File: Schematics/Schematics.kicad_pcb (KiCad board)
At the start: 2 copper layers, 104.1 x 68.6 mm, 15 parts, among them SW1 SW_MEC_5E, U1 74HC595, U2 CC56-12YWA

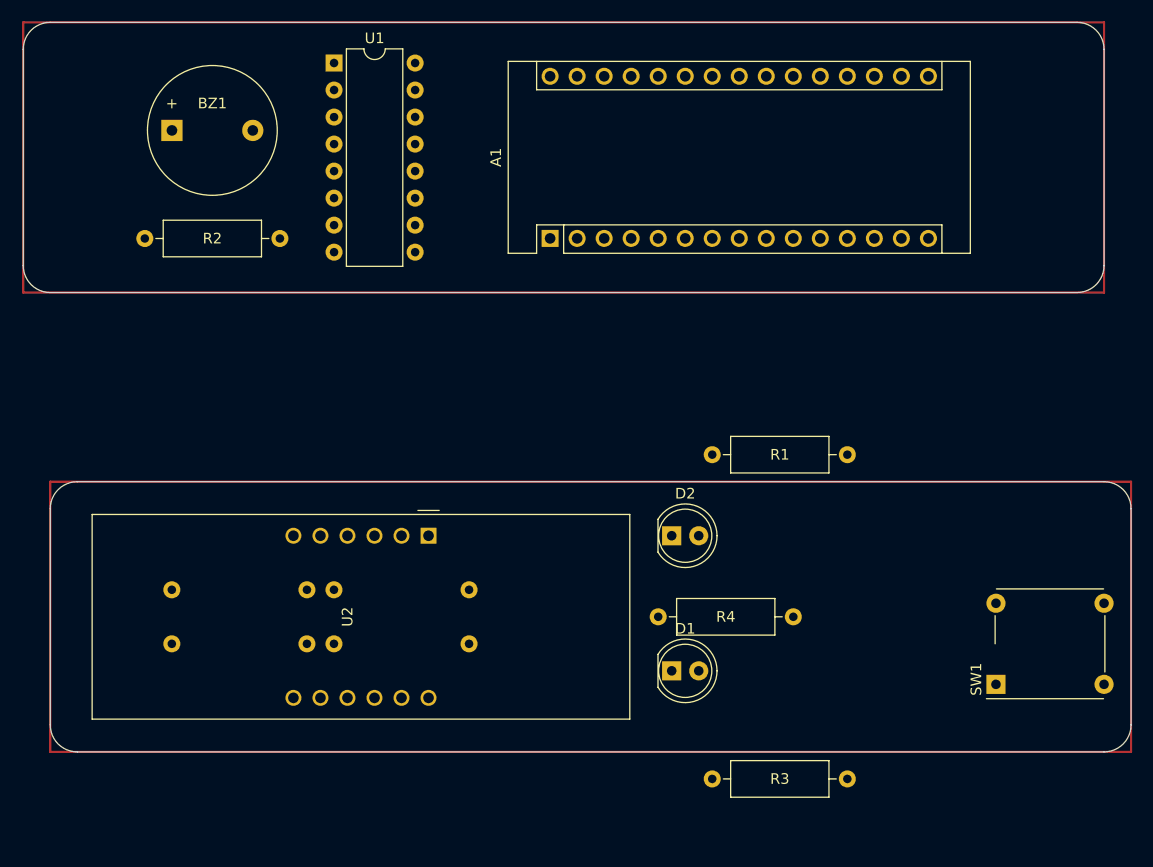
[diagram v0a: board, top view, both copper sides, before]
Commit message: Final Kicad changes
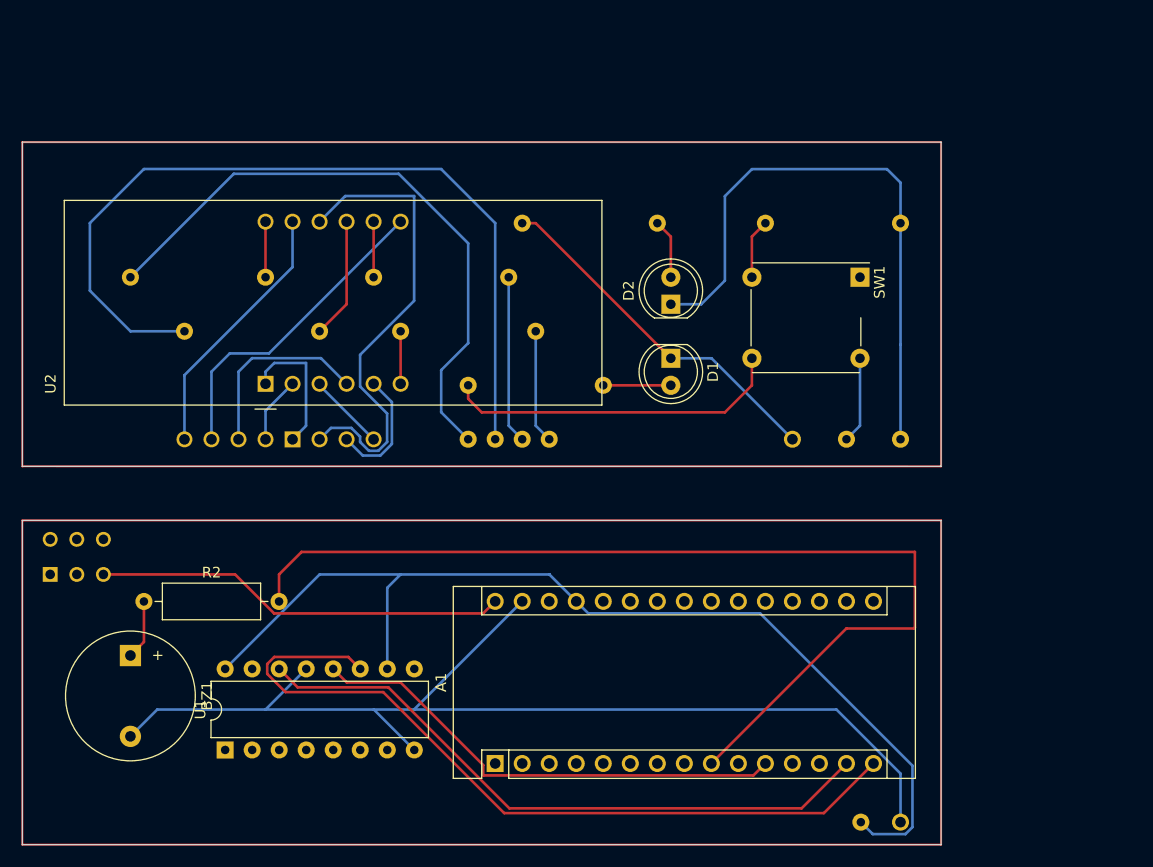
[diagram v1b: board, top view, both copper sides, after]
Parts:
- added ?: , , F.Cu at (121.8, 97.6)
- added ?: , , F.Cu at (143.4, 97.6)
- added ?: , , F.Cu at (140.9, 97.6)
- added ?: , , F.Cu at (166.3, 97.6)
- added ?: , , F.Cu at (171.4, 97.6)
- added ?: , , F.Cu at (176.4, 97.6)
- added ?: , , F.Cu at (172.7, 133.6)
- added ?: , , F.Cu at (138.3, 97.6)
- added ?: , , F.Cu at (135.8, 97.6)
- added ?: , , F.Cu at (109.1, 97.6)
- added ?: , , F.Cu at (116.8, 97.6)
- added ?: , , F.Cu at (176.4, 133.6)
- added ?: , , F.Cu at (111.7, 97.6)
- added ?: , , F.Cu at (119.3, 97.6)
- added ?: , , F.Cu at (114.2, 97.6)
- added ?: , , F.Cu at (124.4, 97.6)
- added ?: , , F.Cu at (126.9, 97.6)
- added SW2: SW_DPDT_x2, Button_Switch_THT:SW_CuK_JS202011CQN_DPDT_Straight, B.Cu at (96.5, 110.3)
- D1: value Green LED -> Green
- D2: value Orange LED -> Orange
- R1, R3, R4: moved to B.Cu
- moved U1 65.4 mm to (113.0, 126.8), turned to 90 degrees
- moved A1 49.6 mm to (138.3, 128.1)
- moved BZ1 49.5 mm to (104.1, 117.9), turned to -90 degrees
- moved SW1 40.3 mm to (172.6, 82.4), turned to -90 degrees
- moved R3 38.4 mm to (148.5, 92.5), turned to 180 degrees
- moved R8 38.2 mm to (104.1, 82.4), turned to 0 degrees
- moved R4 37.0 mm to (153.6, 77.3), turned to 180 degrees
- moved R7 34.7 mm to (139.6, 82.4)
- moved R2 34.1 mm to (105.3, 112.9)
- moved D1 29.4 mm to (154.9, 90.0), turned to -90 degrees
- moved R6 25.1 mm to (142.2, 87.5)
- moved R5 24.3 mm to (109.1, 87.5)
- moved R1 22.3 mm to (163.7, 77.3)
- moved D2 21.8 mm to (154.9, 84.9), turned to 90 degrees
- moved U2 20.9 mm to (116.8, 92.4), turned to 90 degrees
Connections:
- net Net-(A1-Pad5) renamed Dat1
- net Net-(A1-Pad6) renamed Dat2
- net Net-(A1-Pad7) renamed Dat3
- net Net-(A1-Pad8) renamed Dat4
- A1 pad 29: GND -> BT GND
- A1 pad 30: +9V -> Net-(A1-Pad30)
- A1 pad 4: Net-(A1-Pad4) -> unconnected-(A1-Pad4)
- D2 pad 1: Net-(A1-Pad4) -> GND
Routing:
- net GND: track 0.00 -> 161.8 mm
- net Net-(A1-Pad27): track 0.00 -> 136.7 mm
- net Net-(A1-Pad9): track 0.00 -> 94.7 mm
- net Dat2: track 0.00 -> 79.5 mm
- net SRCLK: track 0.00 -> 74.8 mm
- net SER: track 0.00 -> 60.5 mm
- net Dat1: track 0.00 -> 59.0 mm
- net RCLK: track 0.00 -> 45.8 mm
- net Net-(U1-Pad5): track 0.00 -> 44.5 mm
- net Net-(A1-Pad30): track 0.00 -> 38.8 mm
- net Net-(A1-Pad12): track 0.00 -> 33.8 mm
- net Net-(U1-Pad1): track 0.00 -> 30.0 mm
- net Net-(U1-Pad15): track 0.00 -> 24.7 mm
- net Net-(U1-Pad2): track 0.00 -> 18.0 mm
- net Dat3: track 0.00 -> 15.8 mm
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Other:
- board size 104.1 x 68.6 mm -> 86.4 x 66 mm
- board text added: "15-1-2022"
- board text added: "Pomodoro Device"
